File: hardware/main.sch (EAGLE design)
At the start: 30 parts, among them J1 POWER_JACKPTH_BREAD, M1 SERVO, M2 SERVO, M3 SERVO, X1 STEREOJACK

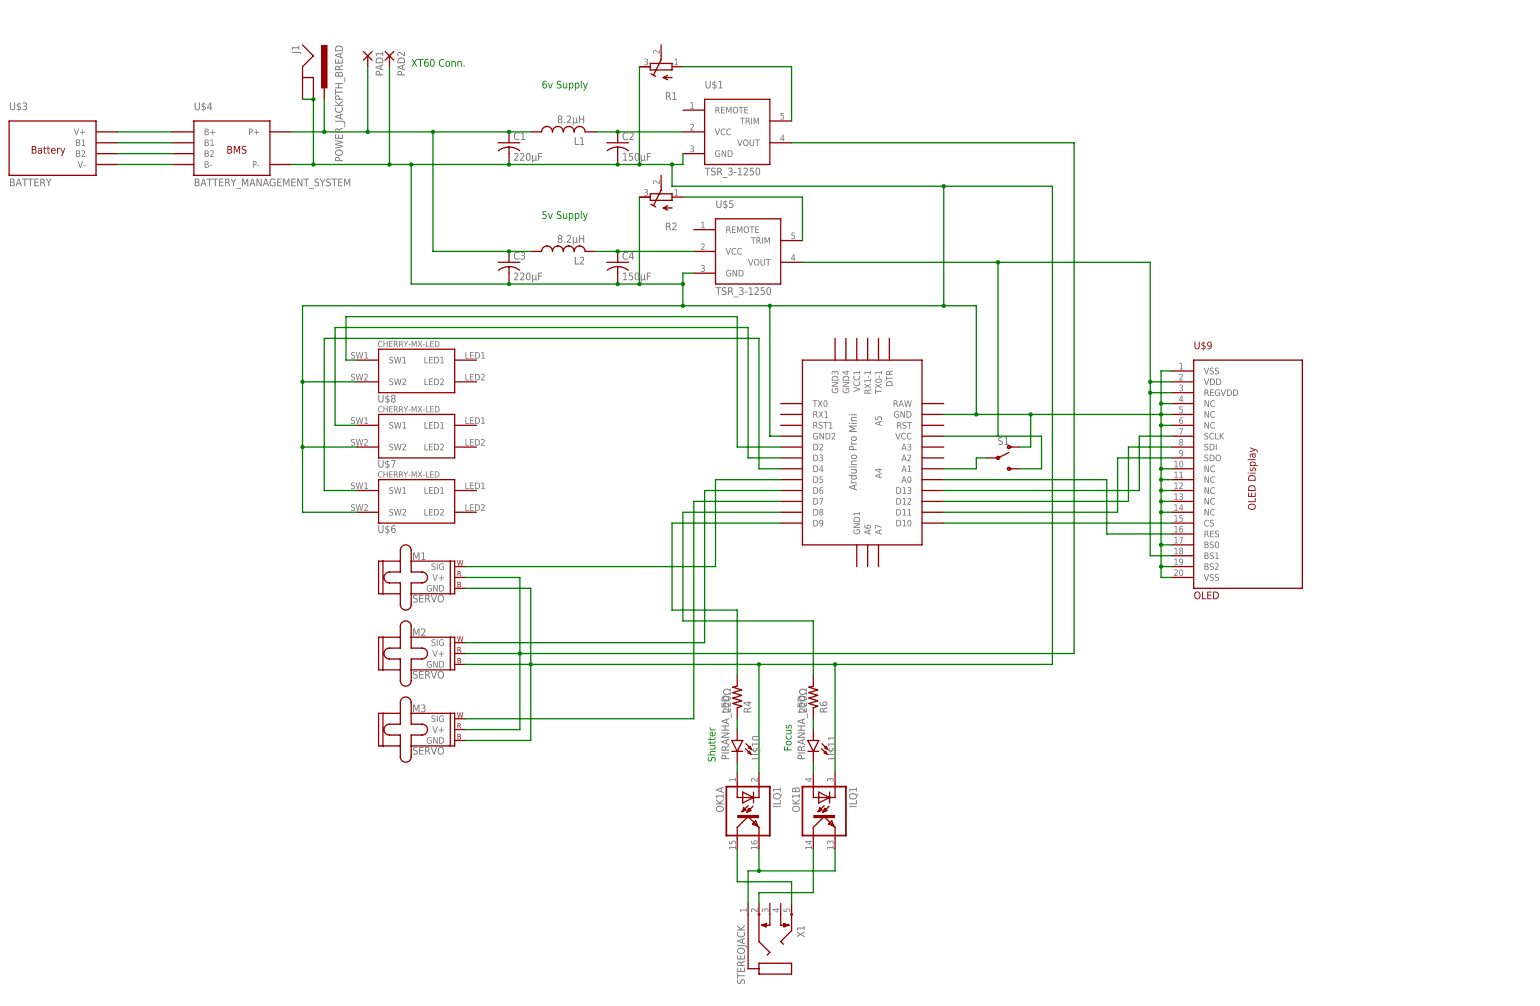
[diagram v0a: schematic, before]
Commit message: Updated hardware
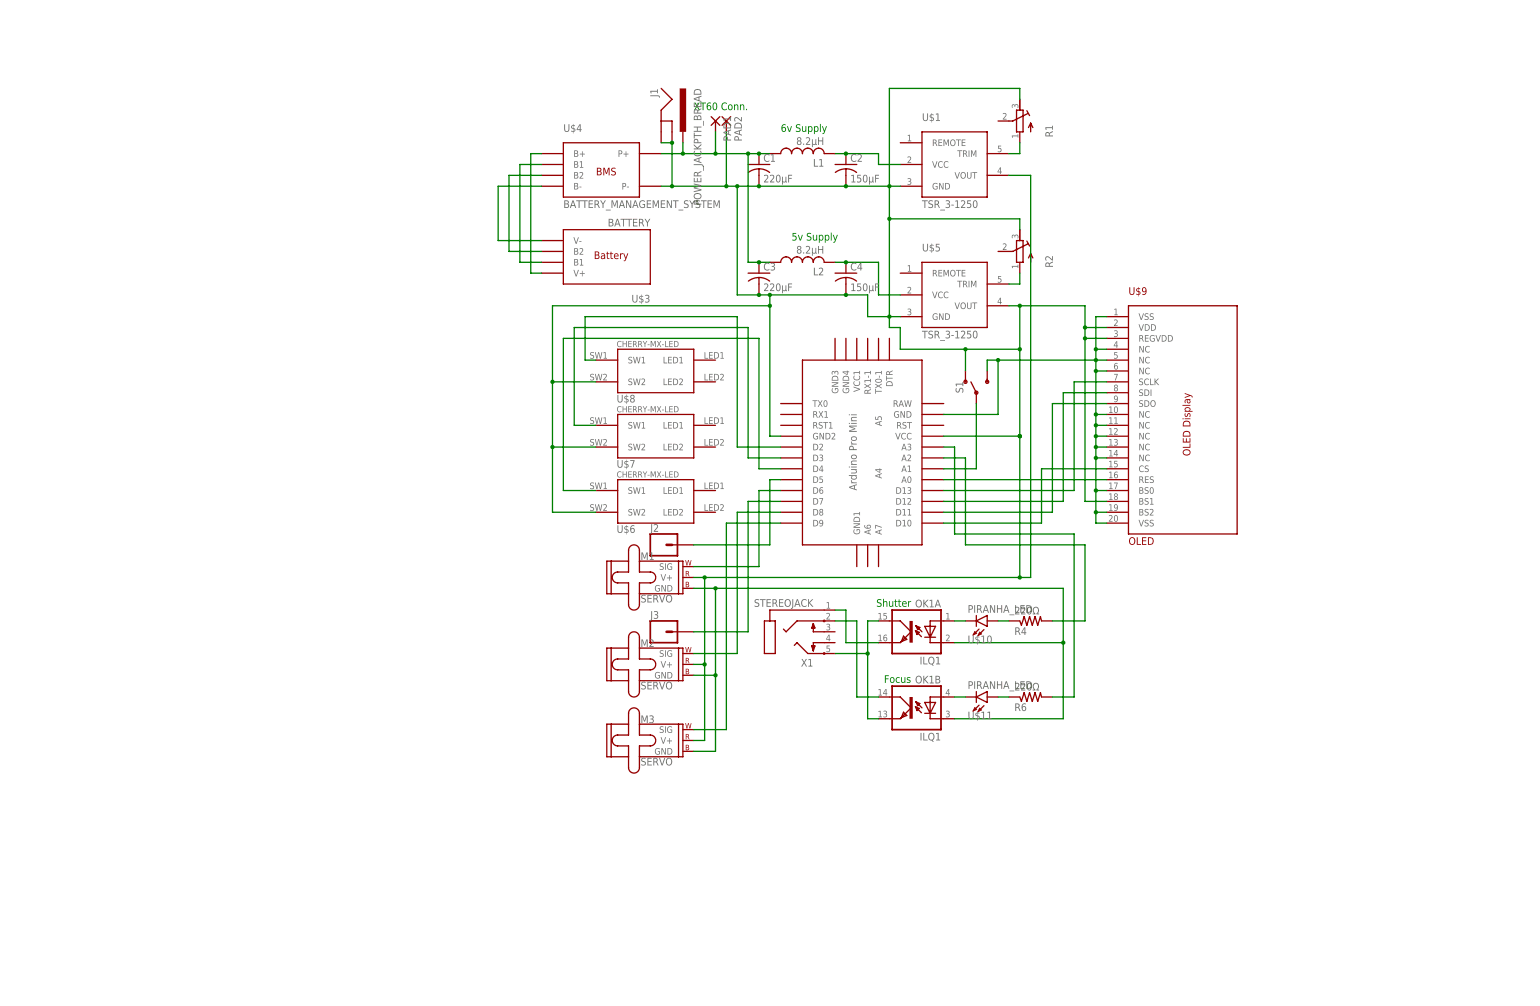
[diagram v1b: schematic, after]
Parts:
- added J2, J3: (no value), SparkFun-Connectors:CONN_01
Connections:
- removed net N$19 (its old number): U$1.VOUT
- removed net N$23: M1.V+, M2.V+, M3.V+
- removed net N$38: C1.2, C2.2, C3.2, C4.2, J1.GND, J1.GNDBREAK, M1.GND, M2.GND, M3.GND, OK1B.C, PAD2.P, R1.E, R2.E, S1.O, U$1.GND, U$2.GND, U$2.GND2, U$4.P-, U$5.GND, U$6.SW2, U$7.SW2, U$8.SW2, U$9.BS0, U$9.BS2, U$9.NC@0, U$9.NC@1, U$9.NC@2, U$9.NC@3, U$9.NC@4, U$9.NC@5, U$9.NC@6, U$9.NC@7, U$9.VSS@0, U$9.VSS@1
- removed net N$42: S1.S, U$2.VCC, U$5.VOUT, U$9.BS1, U$9.REGVDD, U$9.VDD
- new net N$20: M2.SIG, U$2.D8
- new net N$28: M3.SIG, U$2.D9
- new net N$37: S1.S, U$2.GND, U$9.BS0, U$9.BS2, U$9.NC@0, U$9.NC@1, U$9.NC@2, U$9.NC@3, U$9.NC@4, U$9.NC@5, U$9.NC@6, U$9.NC@7, U$9.VSS@0, U$9.VSS@1
- new net N$4: C1.2, C2.2, C3.2, C4.2, J1.GND, J1.GNDBREAK, M1.V+, M2.V+, M3.V+, PAD2.P, R1.E, R2.E, S1.O, U$1.GND, U$1.VOUT, U$2.GND2, U$2.VCC, U$4.P-, U$5.GND, U$5.VOUT, U$6.SW2, U$7.SW2, U$8.SW2, U$9.BS1, U$9.REGVDD, U$9.VDD
- net N$11: now also J2.1; no longer M1.SIG
- net N$16: now also M1.SIG; no longer M2.SIG
- net N$17: now also J3.1; no longer M3.SIG
- net N$30: now also R4.2, U$2.A2; no longer R6.2, U$2.D8
- net N$31: now also R6.2, U$2.A3; no longer R4.2, U$2.D9
- net N$32: now also M1.GND, M2.GND, M3.GND, OK1B.C
- net N$33: now also OK1B.EMIT
- net N$34: no longer OK1B.EMIT
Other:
- moved on the sheet: C1, C2, C3, C4, J1, L1, L2, M1, M2, M3, OK1A, OK1B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

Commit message: Cleaned up schematic and board layout
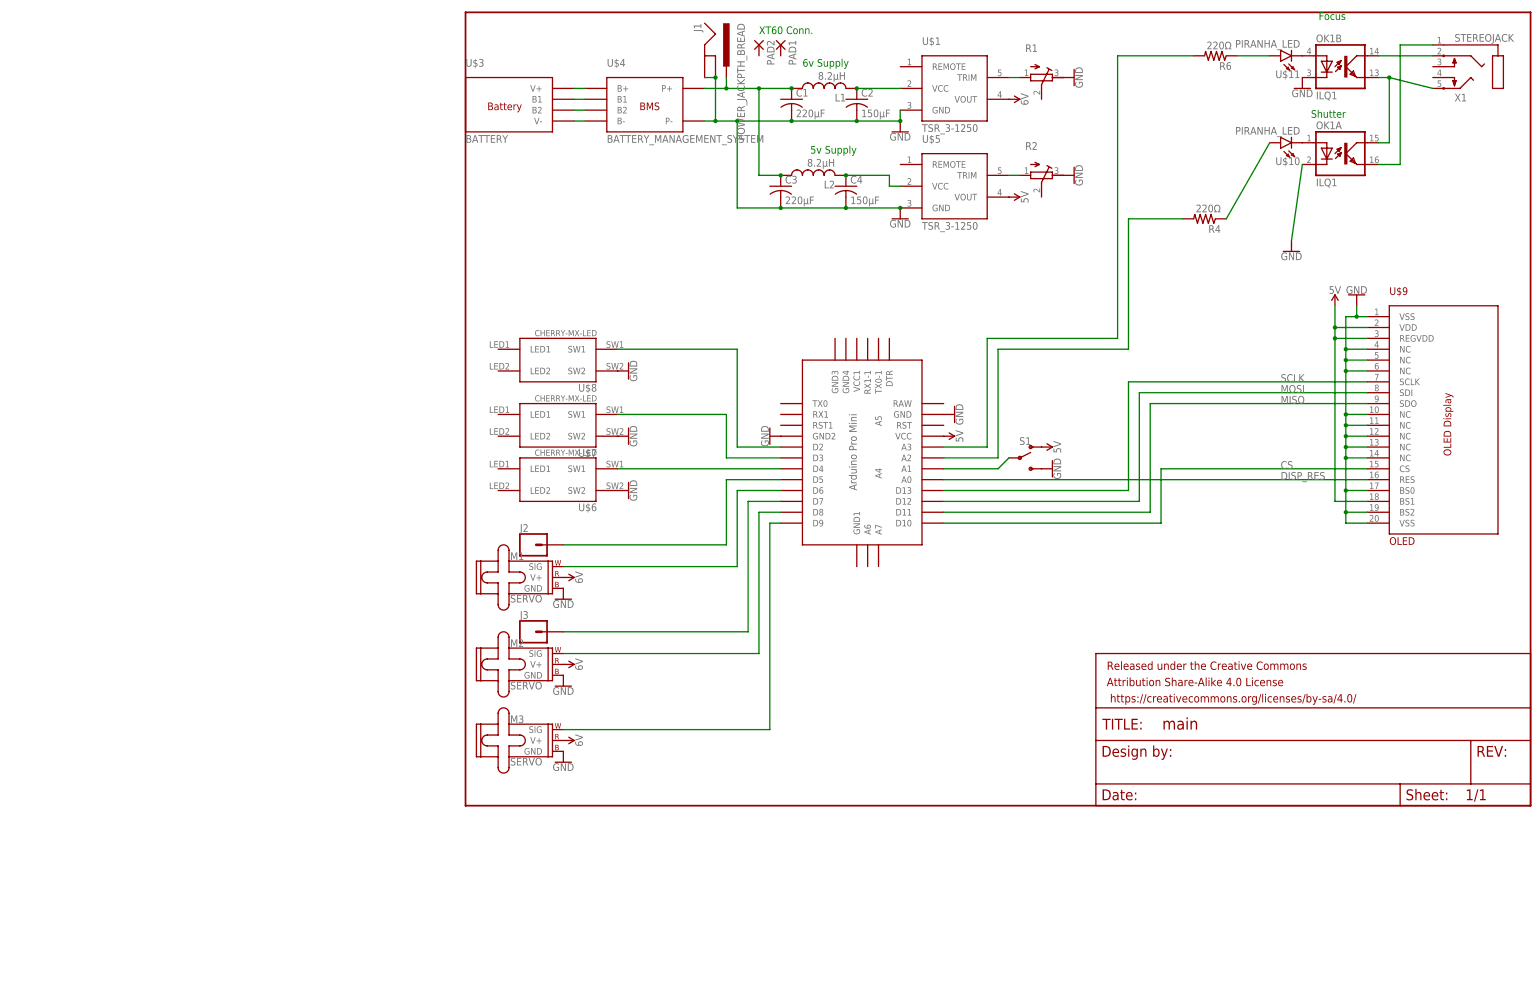
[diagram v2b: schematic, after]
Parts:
- added FRAME1: FRAME-LETTER, SparkFun-Aesthetics:FRAME-LETTER
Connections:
- net N$11 renamed SERVO_1_FEEDBACK
- net N$12 renamed BUTTON_3
- net N$13 renamed BUTTON_1
- net N$14 renamed BUTTON_2
- net N$15 renamed MODE_SWITCH
- net N$16 renamed SERVO_1_CONTROL
- net N$17 renamed SERVO_2_FEEDBACK
- net N$18 renamed MOSI
- net N$19 renamed DISP_RES
- net N$20 renamed SERVO_2_CONTROL
- net N$21 renamed MISO
- net N$22 renamed CS
- net N$25 renamed SCLK
- net N$28 renamed SERVO_3_CONTROL
- net N$30 renamed SHUTTER
- net N$31 renamed FOCUS
- removed net N$32: M1.GND, M2.GND, M3.GND, OK1A.C, OK1B.C
- removed net N$37: S1.S, U$2.GND, U$9.BS0, U$9.BS2, U$9.NC@0, U$9.NC@1, U$9.NC@2, U$9.NC@3, U$9.NC@4, U$9.NC@5, U$9.NC@6, U$9.NC@7, U$9.VSS@0, U$9.VSS@1
- removed net N$4 (its old number): C1.2, C2.2, C3.2, C4.2, J1.GND, J1.GNDBREAK, M1.V+, M2.V+, M3.V+, PAD2.P, R1.E, R2.E, S1.O, U$1.GND, U$1.VOUT, U$2.GND2, U$2.VCC, U$4.P-, U$5.GND, U$5.VOUT, U$6.SW2, U$7.SW2, U$8.SW2, U$9.BS1, U$9.REGVDD, U$9.VDD
- removed net N$5 (its old number): C1.1, C3.1, J1.PWR, L1.1, L2.1, PAD1.P, U$4.P+
- new net 5V: S1.O, U$2.VCC, U$5.VOUT, U$9.BS1, U$9.REGVDD, U$9.VDD
- new net 6V: M1.V+, M2.V+, M3.V+, U$1.VOUT
- new net GND: C1.2, C2.2, C3.2, C4.2, J1.GND, J1.GNDBREAK, M1.GND, M2.GND, M3.GND, OK1A.C, OK1B.C, R1.E, R2.E, S1.S, U$1.GND, U$2.GND, U$2.GND2, U$4.P-, U$5.GND, U$6.SW2, U$7.SW2, U$8.SW2, U$9.BS0, U$9.BS2, U$9.NC@0, U$9.NC@1, U$9.NC@2, U$9.NC@3, U$9.NC@4, U$9.NC@5, U$9.NC@6, U$9.NC@7, U$9.VSS@0, U$9.VSS@1
- new net P+: C1.1, C3.1, J1.PWR, L1.1, L2.1, U$4.P+
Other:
- moved on the sheet: C1, C2, C3, C4, J1, J2, J3, L1, L2, M1, M2, M3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
